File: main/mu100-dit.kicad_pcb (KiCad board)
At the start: 2 copper layers, 18 x 40 mm, 22 parts, among them J1 Conn_01x10_Female, J2 Conn_01x02_Male, U1 TOTX-177L, U2 AK4103A, U3 APX809S-46SR-7

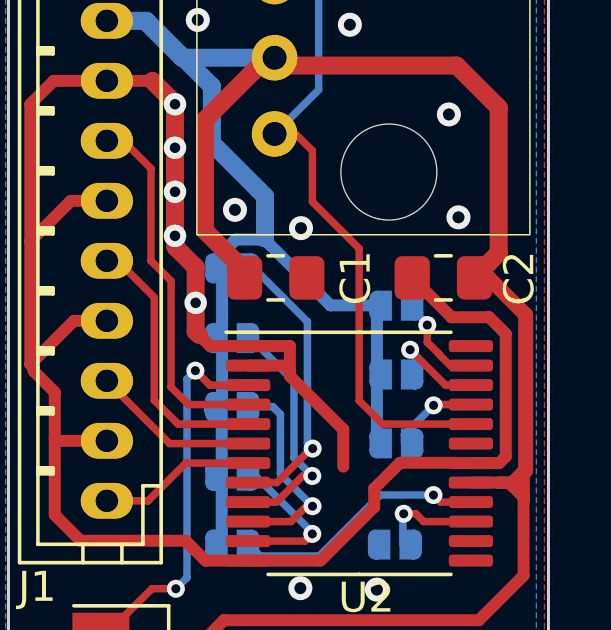
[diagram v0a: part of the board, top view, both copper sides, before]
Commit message: minor tweaks to main board
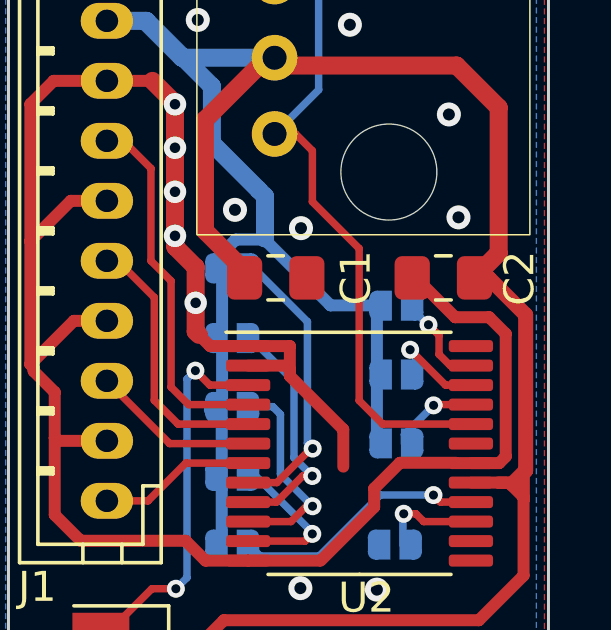
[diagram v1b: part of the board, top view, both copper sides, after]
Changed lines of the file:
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@@
   )
   (segment (start 82.55 94.572) (end 83.3 95.322) (width 0.6) (layer "F.Cu") (net 1))
-  (segment (start 92.5205 102.452) (end 91.2085 101.14) (width 0.4) (layer "F.Cu") (net 1))
   (segment (start 83.3 95.352) (end 83.3 99.7386) (width 0.6) (layer "F.Cu") (net 1))
   (segment (start 83.655 109.902) (end 80.155 109.902) (width 0.4) (layer "F.Cu") (net 1))
+  (segment (start 94.32548 107.09652) (end 94.32548 103.00248) (width 0.4) (layer "F.Cu") (net 1))
   (segment (start 86.991427 104.063427) (end 87.13 104.202) (width 0.4) (layer "F.Cu") (net 1))
+  (segment (start 93.1645 107.313427) (end 94.108573 107.313427) (width 0.4) (layer "F.Cu") (net 1))
   (segment (start 88.118573 110.563427) (end 85.7395 110.563427) (width 0.4) (layer "F.Cu") (net 1))
   (segment (start 85.7395 103.413427) (end 87.13 103.413427) (width 0.4) (layer "F.Cu") (net 1))
   (segment (start 78.588 104.246) (end 79.292 104.95) (width 0.4) (layer "F.Cu") (net 1))
   (segment (start 89.94 108.78) (end 89.94 108.162) (width 0.4) (layer "F.Cu") (net 1))
-  (segment (start 93.775 102.452) (end 92.5205 102.452) (width 0.4) (layer "F.Cu") (net 1))
   (segment (start 81.03 98.572) (end 79.828 98.572) (width 0.4) (layer "F.Cu") (net 1))
   (segment (start 78.48 99.92) (end 78.48 104.022) (width 0.4) (layer "F.Cu") (net 1))
@@
   (segment (start 83.99 101.972) (end 83.99 100.78601) (width 0.6) (layer "F.Cu") (net 1))
   (segment (start 79.292 109.039) (end 79.292 106.474) (width 0.4) (layer "F.Cu") (net 1))
-  (segment (start 94.32548 107.09652) (end 94.32548 103.00248) (width 0.4) (layer "F.Cu") (net 1))
   (segment (start 83.99 102.9306) (end 83.99 101.972) (width 0.6) (layer "F.Cu") (net 1))
   (segment (start 83.99 100.78601) (end 83.3126 100.10861) (width 0.6) (layer "F.Cu") (net 1))
   (segment (start 88.156573 110.563427) (end 89.94 108.78) (width 0.4) (layer "F.Cu") (net 1))
-  (segment (start 94.32548 103.00248) (end 93.775 102.452) (width 0.4) (layer "F.Cu") (net 1))
   (segment (start 81.03 94.572) (end 79.256 94.572) (width 0.4) (layer "F.Cu") (net 1))
   (segment (start 81.03 94.572) (end 82.55 94.572) (width 0.4) (layer "F.Cu") (net 1))
@@
   (segment (start 84.1 103.0406) (end 83.99 102.9306) (width 0.6) (layer "F.Cu") (net 1))
   (segment (start 85.7395 110.563427) (end 84.316427 110.563427) (width 0.4) (layer "F.Cu") (net 1))
+  (segment (start 94.32548 103.00248) (end 93.775 102.452) (width 0.4) (layer "F.Cu") (net 1))
+  (segment (start 94.108573 107.313427) (end 94.32548 107.09652) (width 0.4) (layer "F.Cu") (net 1))
   (segment (start 85.7395 104.063427) (end 86.991427 104.063427) (width 0.4) (layer "F.Cu") (net 1))
-  (segment (start 94.108573 107.313427) (end 94.32548 107.09652) (width 0.4) (layer "F.Cu") (net 1))
+  (segment (start 92.64 102.452) (end 91.328 101.14) (width 0.4) (layer "F.Cu") (net 1))
   (segment (start 78.48 104.022) (end 78.588 104.13) (width 0.4) (layer "F.Cu") (net 1))
   (segment (start 87.13 104.412) (end 88.91 106.192) (width 0.4) (layer "F.Cu") (net 1))
@@
   (segment (start 83.3126 100.10861) (end 83.3126 99.7132) (width 0.6) (layer "F.Cu") (net 1))
   (segment (start 87.13 104.202) (end 87.13 104.412) (width 0.4) (layer "F.Cu") (net 1))
+  (segment (start 91.328 101.14) (end 91.2085 101.14) (width 0.4) (layer "F.Cu") (net 1))
   (segment (start 79.292 104.95) (end 79.292 106.474) (width 0.4) (layer "F.Cu") (net 1))
   (segment (start 82.343 81.702) (end 80.91 83.135) (width 0.4) (layer "F.Cu") (net 1))
+  (segment (start 93.775 102.452) (end 92.64 102.452) (width 0.4) (layer "F.Cu") (net 1))
   (segment (start 80.155 109.902) (end 79.292 109.039) (width 0.4) (layer "F.Cu") (net 1))
   (segment (start 79.93 102.572) (end 78.48 104.022) (width 0.4) (layer "F.Cu") (net 1))
   (segment (start 78.48 95.348) (end 78.48 99.92) (width 0.4) (layer "F.Cu") (net 1))
   (segment (start 83.3 95.322) (end 83.3 95.352) (width 0.6) (layer "F.Cu") (net 1))
-  (segment (start 93.1645 107.313427) (end 94.108573 107.313427) (width 0.4) (layer "F.Cu") (net 1))
   (segment (start 87.13 103.413427) (end 87.13 104.202) (width 0.4) (layer "F.Cu") (net 1))
   (segment (start 89.94 108.162) (end 90.798573 107.303427) (width 0.4) (layer "F.Cu") (net 1))
@@
   (segment (start 91.138872 103.534614) (end 91.32 103.715742) (width 0.25) (layer "B.Cu") (net 14))
   (segment (start 91.32 103.715742) (end 91.32 104.352) (width 0.25) (layer "B.Cu") (net 14))
-  (segment (start 91.71 102.712) (end 91.71 103.282) (width 0.25) (layer "F.Cu") (net 15))
-  (segment (start 91.71 103.282) (end 92.10248 103.67448) (width 0.25) (layer "F.Cu") (net 15))
   (segment (start 92.10248 103.689268) (end 92.476639 104.063427) (width 0.25) (layer "F.Cu") (net 15))
-  (segment (start 92.10248 103.67448) (end 92.10248 103.689268) (width 0.25) (layer "F.Cu") (net 15))
+  (segment (start 92.10248 103.05448) (end 92.10248 103.689268) (width 0.25) (layer "F.Cu") (net 15))
+  (segment (start 91.75 102.702) (end 92.10248 103.05448) (width 0.25) (layer "F.Cu") (net 15))
   (segment (start 92.476639 104.063427) (end 93.1645 104.063427) (width 0.25) (layer "F.Cu") (net 15))
-  (via (at 91.71 102.712) (size 0.6) (drill 0.3) (layers "F.Cu" "B.Cu") (free) (net 15))
-  (segment (start 91.71 102.712) (end 91.71 102.682) (width 0.25) (layer "B.Cu") (net 15))
-  (segment (start 91.71 102.682) (end 91.085 102.057) (width 0.25) (layer "B.Cu") (net 15))
+  (via (at 91.75 102.702) (size 0.6) (drill 0.3) (layers "F.Cu" "B.Cu") (free) (net 15))
+  (segment (start 91.73 102.702) (end 91.085 102.057) (width 0.25) (layer "B.Cu") (net 15))
+  (segment (start 91.75 102.702) (end 91.73 102.702) (width 0.25) (layer "B.Cu") (net 15))
   (segment (start 91.3315 109.0035) (end 91.591427 109.263427) (width 0.25) (layer "F.Cu") (net 16))
   (segment (start 90.9252 109.0035) (end 91.3315 109.0035) (width 0.25) (layer "F.Cu") (net 16))
